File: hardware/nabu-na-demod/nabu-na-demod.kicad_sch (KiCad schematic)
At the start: 38 parts, among them U2 74LS74, U3 74LS74, U4 74LS86, U6 74LS86, U7 74LS00

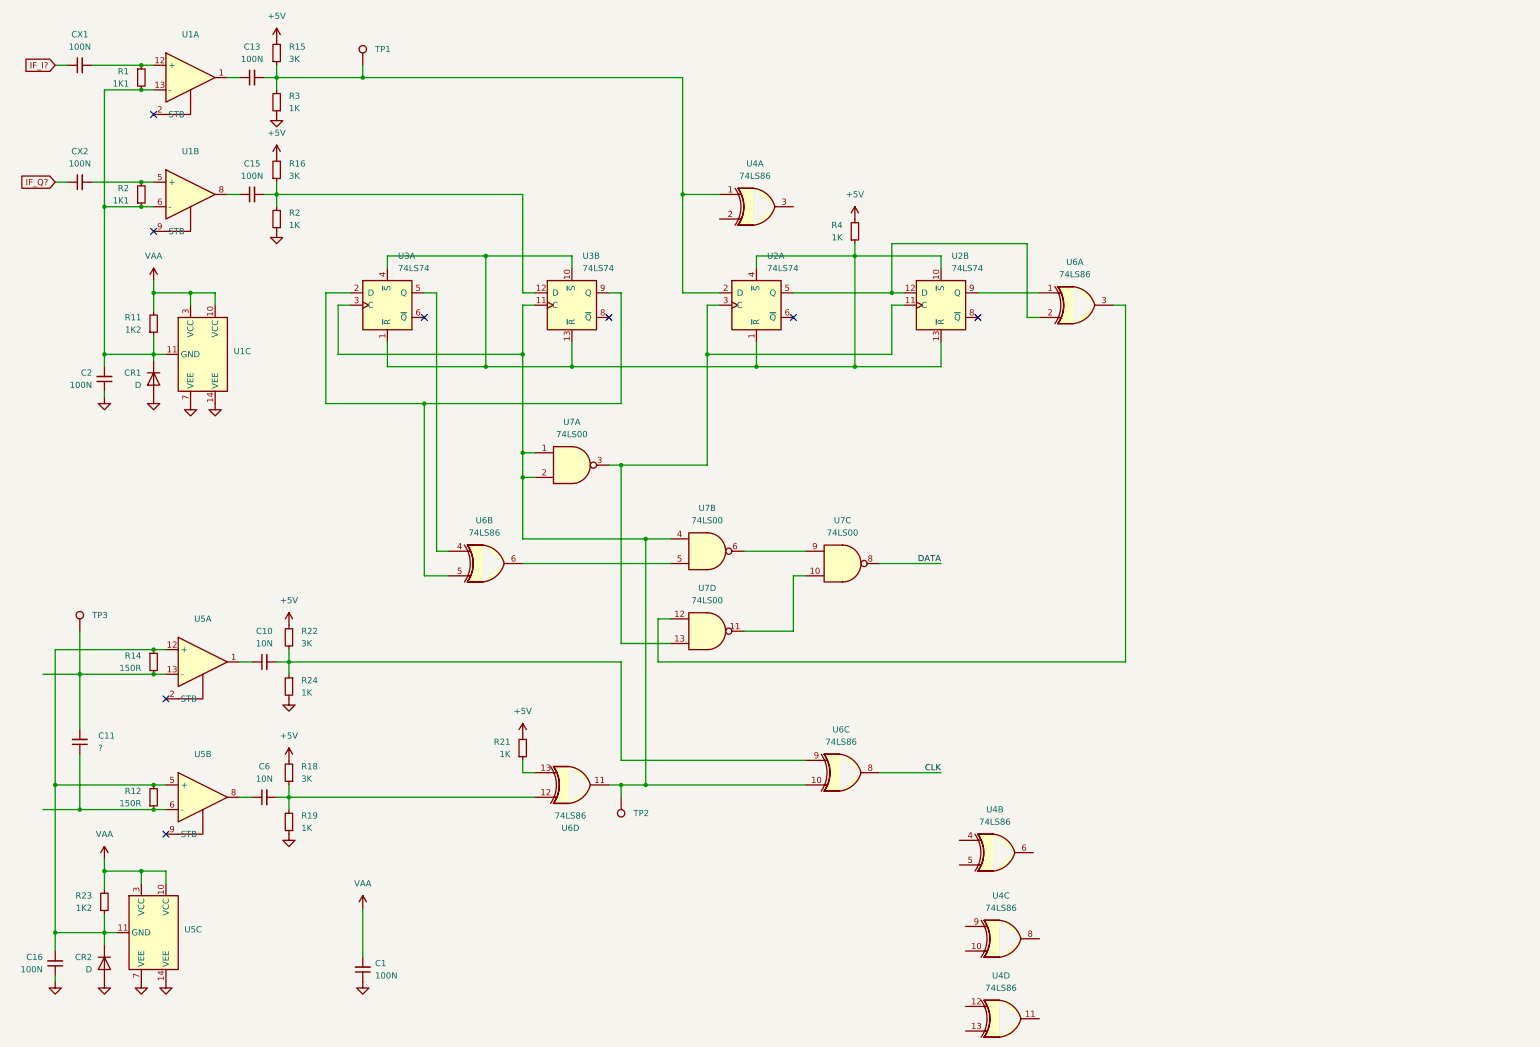
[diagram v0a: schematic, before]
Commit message: Clean up demodulator schematic -- still incomplete!
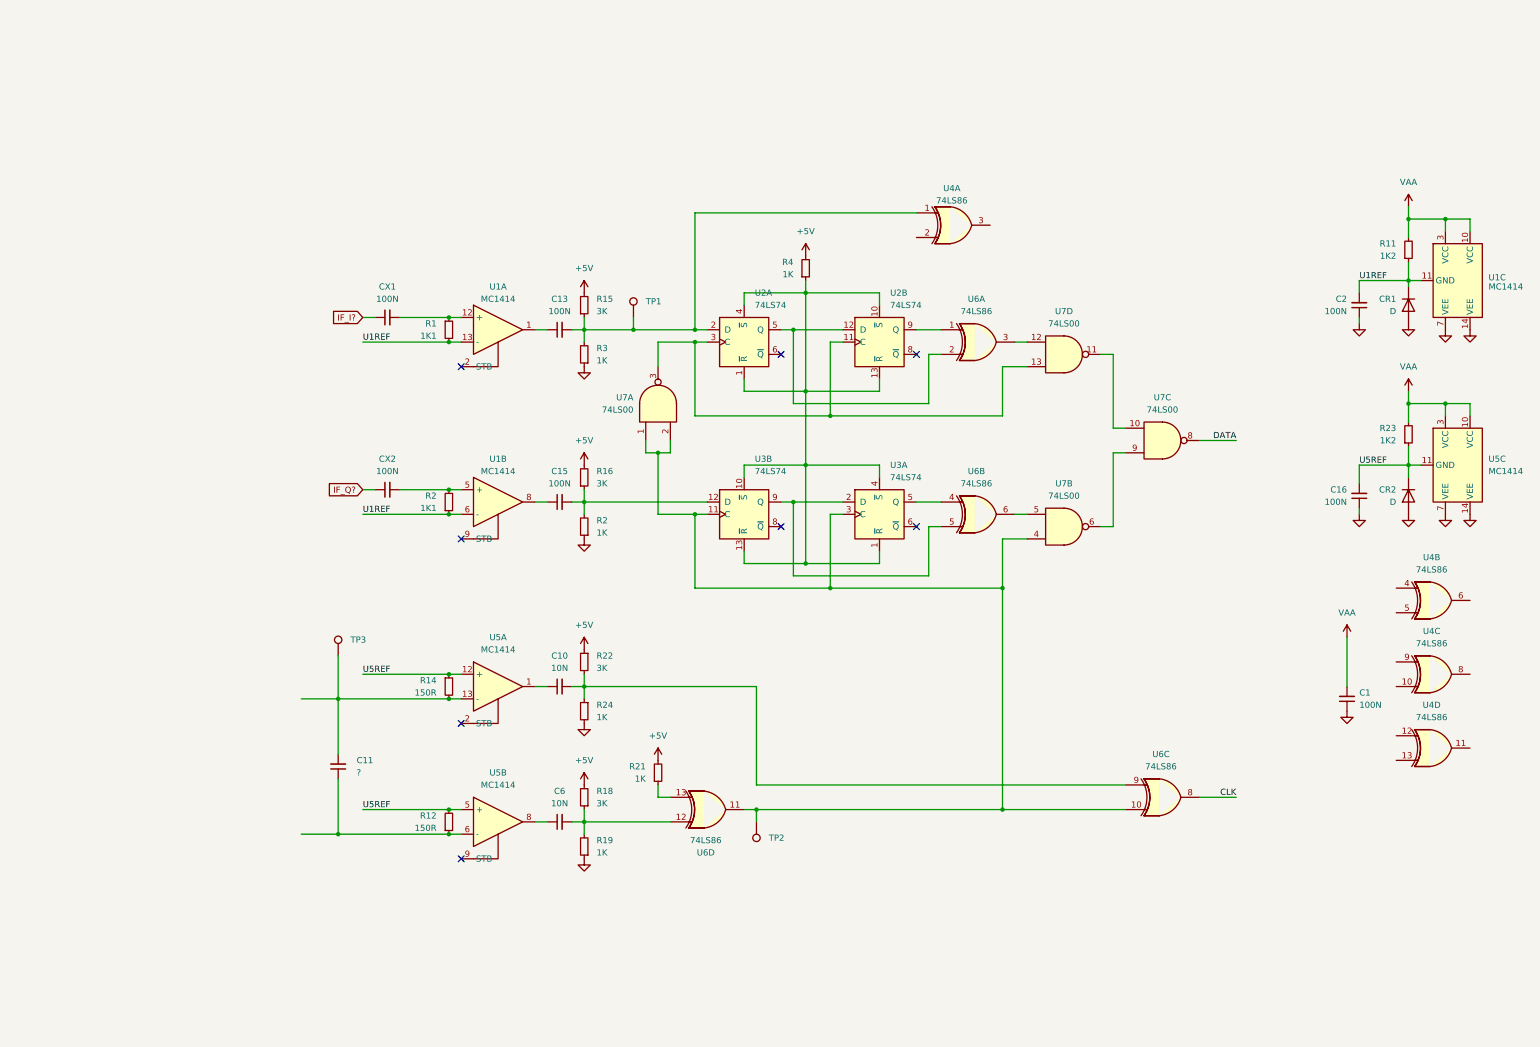
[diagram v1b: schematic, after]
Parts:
- U1, U5: value ~ -> MC1414
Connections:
- net U1REF: now reaches C2.2, CR1.1 (K), R1.2, R11.1, R2.1, U1.11 (GND), U1.13 (-), U1.6 (-)
- net U5REF: now reaches C16.2, CR2.1 (K), R12.2, R14.1, R23.1, U5.11 (GND), U5.12 (+), U5.5 (+)
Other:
- moved on the sheet: C1, C10, C11, C13, C15, C16, C2, C6, CR1, CR2, CX1, CX2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
